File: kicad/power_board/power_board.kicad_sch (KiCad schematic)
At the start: 58 parts, among them J1 24V, J2 5V, J3 3V3, J4 GND, J6 Grid, J7 MCU, J8 Solar Panel, Q1 FDD8453LZ, Q2 FDD8453LZ, Q3 FDD8453LZ, Q4 FDD8453LZ, Q5 FDS5670, U1 LM2575D2T-3.3R4G, U2 LM2575D2T-5R4G, U5 LT3757A, U6 LT1161

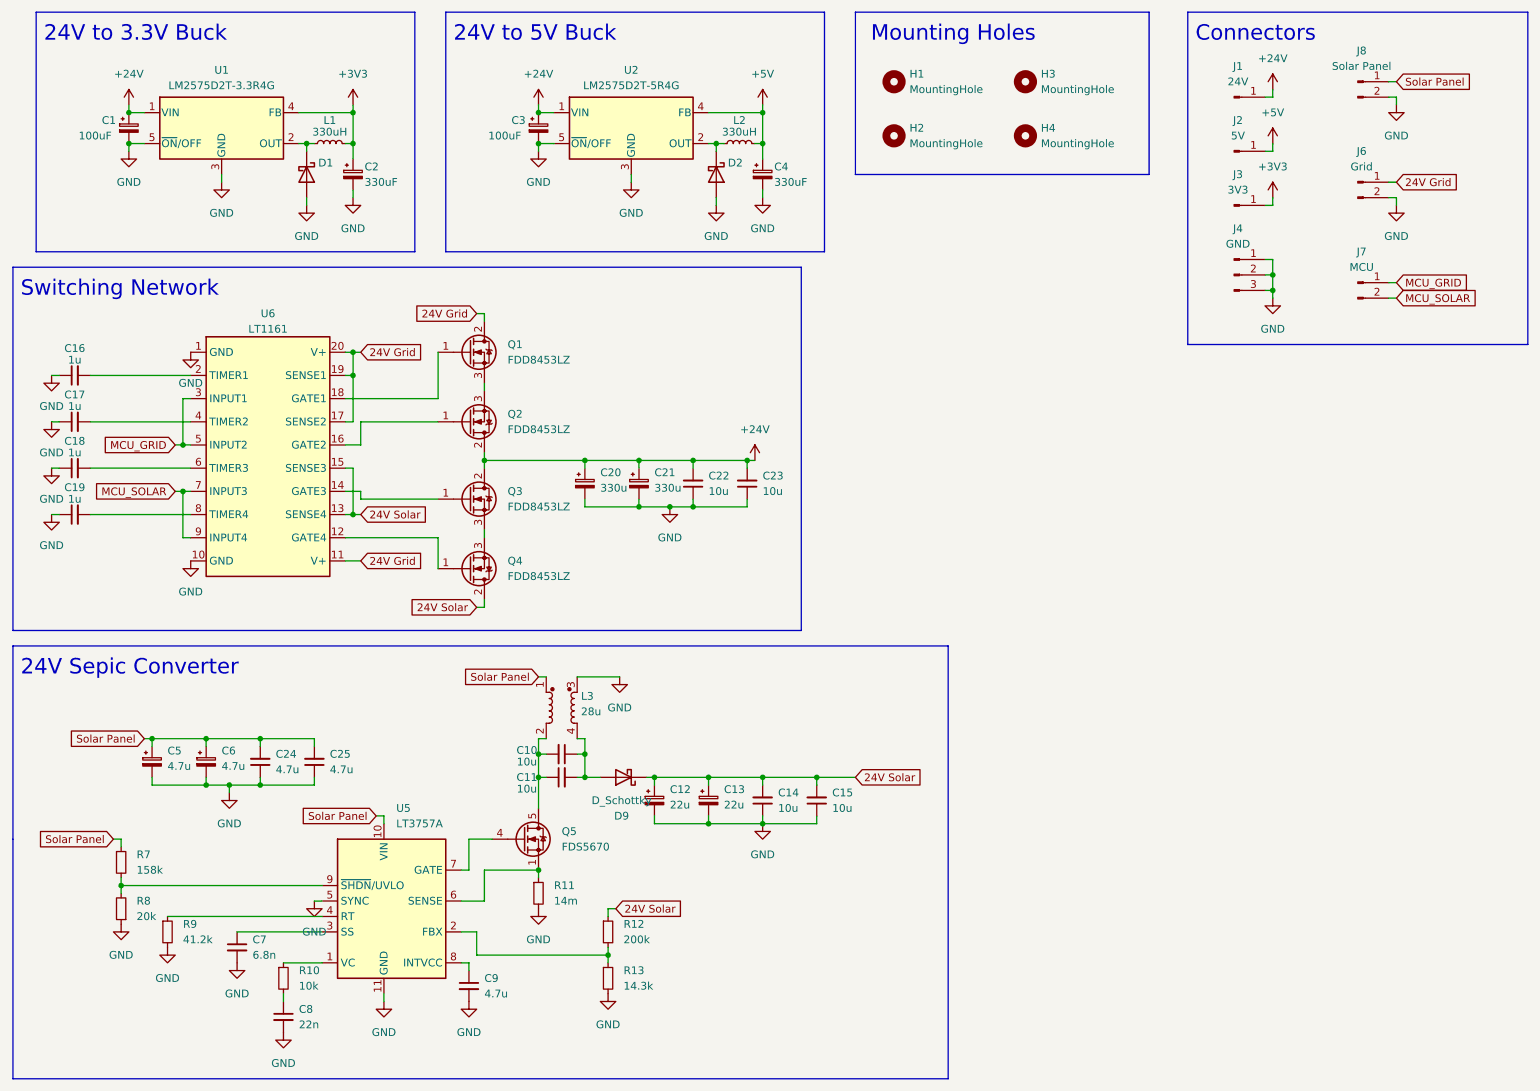
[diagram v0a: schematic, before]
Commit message: traffic lights WIP
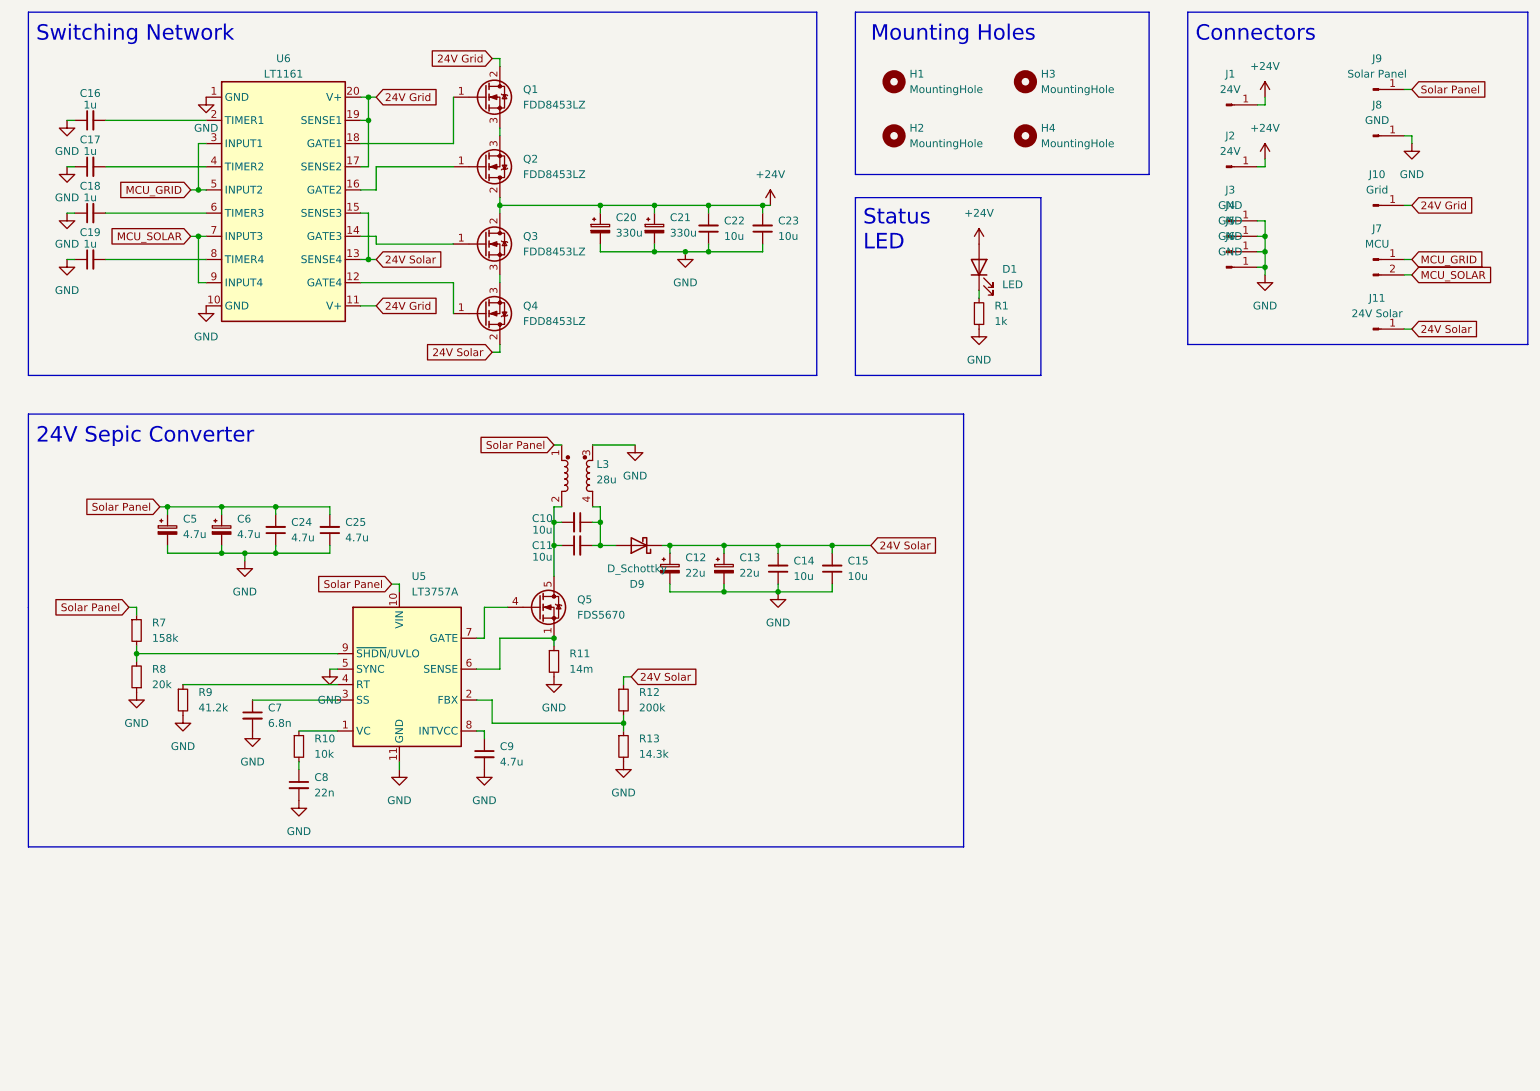
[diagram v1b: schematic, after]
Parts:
- removed C1, C3: 100uF, Capacitor_THT:C_Radial_D8.0mm_H11.5mm_P3.50mm, symbol Device:C_Polarized_Small
- removed C2, C4: 330uF, Capacitor_THT:CP_Radial_D8.0mm_P3.50mm, symbol Device:C_Polarized_Small
- removed D1, D2: VS-30WQ04FNTR-M3, Package_TO_SOT_SMD:TO-252-2, symbol Device:D_Schottky
- removed J4: GND, Connector_PinHeader_2.54mm:PinHeader_1x03_P2.54mm_Vertical, symbol Connector:Conn_01x03_Male
- removed J6: Grid, Connector_PinHeader_2.54mm:PinHeader_1x02_P2.54mm_Vertical, symbol Connector:Conn_01x02_Male
- removed J8: Solar Panel, Connector_PinHeader_2.54mm:PinHeader_1x02_P2.54mm_Vertical, symbol Connector:Conn_01x02_Male
- removed L1, L2: 330uH, Inductor_THT:L_Toroid_Vertical_L31.8mm_W15.9mm_P13.50mm_Bourns_5700, symbol Device:L_Small
- removed U1: LM2575D2T-3.3R4G, Package_TO_SOT_SMD:TO-263-5_TabPin3, symbol Regulator_Switching:LM2575-3.3BU
- removed U2: LM2575D2T-5R4G, Package_TO_SOT_SMD:TO-263-5_TabPin3, symbol Regulator_Switching:LM2575-5.0BU
- added D1: LED, Capacitor_SMD:C_0603_1608Metric, symbol Device:LED
- added J10: Grid, Connector_PinHeader_2.54mm:PinHeader_1x01_P2.54mm_Vertical, symbol Connector:Conn_01x01_Male
- added J11: 24V Solar, Connector_PinHeader_2.54mm:PinHeader_1x01_P2.54mm_Vertical, symbol Connector:Conn_01x01_Male
- added J4, J5, J6: GND, Connector_PinHeader_2.54mm:PinHeader_1x01_P2.54mm_Vertical, symbol Connector:Conn_01x01_Male
- added J8: GND, _mine:73099, symbol Connector:Conn_01x01_Male
- added J9: Solar Panel, _mine:73099, symbol Connector:Conn_01x01_Male
- added R1: 1k, Resistor_SMD:R_2512_6332Metric, symbol Device:R_Small
- J2: value 5V -> 24V
- J3: value 3V3 -> GND
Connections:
- net +3V3 is gone; now on net GND: J3.1 (Pin_1)
- net +5V is gone; now on net +24V: J2.1 (Pin_1)
- net +24V: now also D1.2 (A)
- net 24V Grid: now also J10.1 (Pin_1)
- net 24V Solar: now also J11.1 (Pin_1)
- net GND: now also J4.1 (Pin_1), J5.1 (Pin_1), J6.1 (Pin_1), J8.1 (Pin_1), R1.2
- net Solar Panel: now also J9.1 (Pin_1)
- new net: D1.1 (K), R1.1
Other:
- note added: "Status LED"
- note removed: "24V to 3.3V Buck"
- note removed: "24V to 5V Buck"
- moved on the sheet: C10, C11, C12, C13, C14, C15, C16, C17, C18, C19, C20, C21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
